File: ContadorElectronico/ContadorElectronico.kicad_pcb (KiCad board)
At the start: 2 copper layers, 60 x 90 mm, 24 parts, among them J1 INPUT, J2 POWER, SW1 MODE, SW2 INC, SW3 DEC, U1 LM358, U3 4N35, U4 4N35

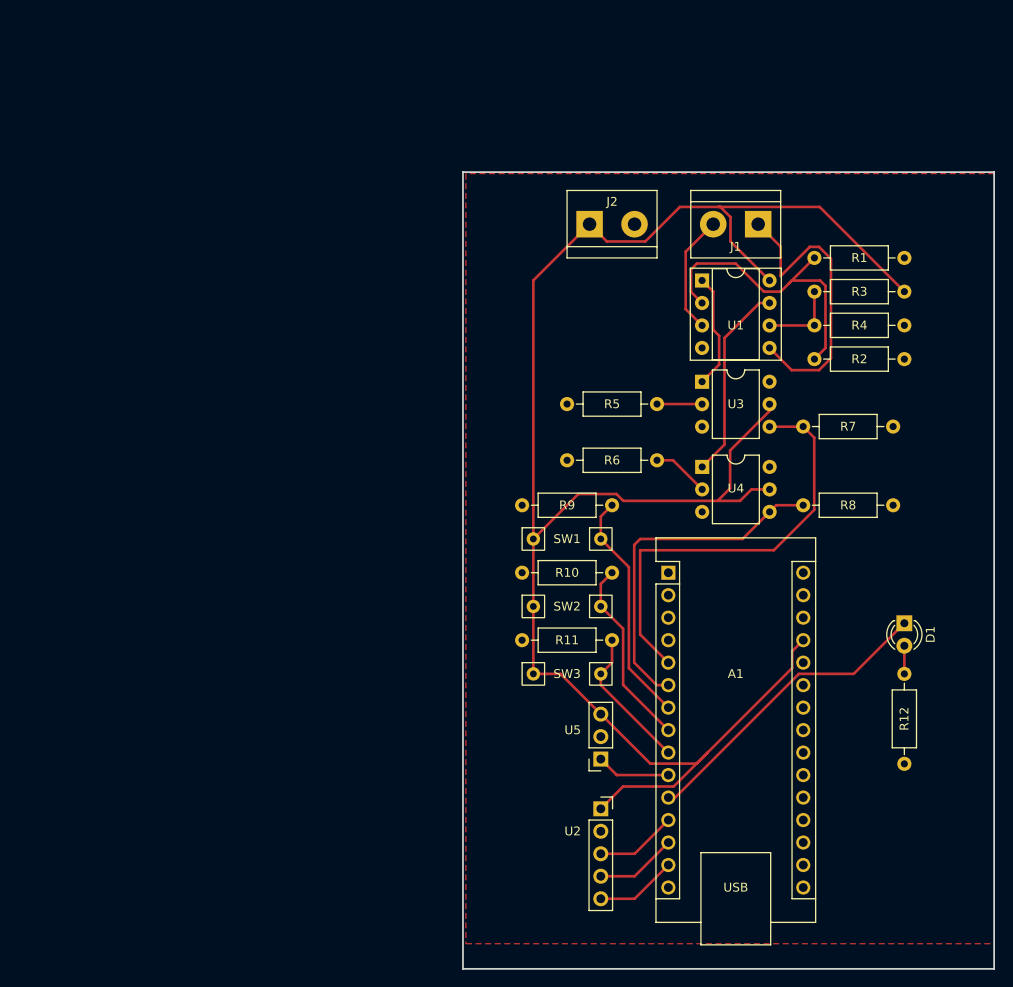
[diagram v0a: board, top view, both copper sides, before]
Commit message: PCB con tolerancias adecuadas
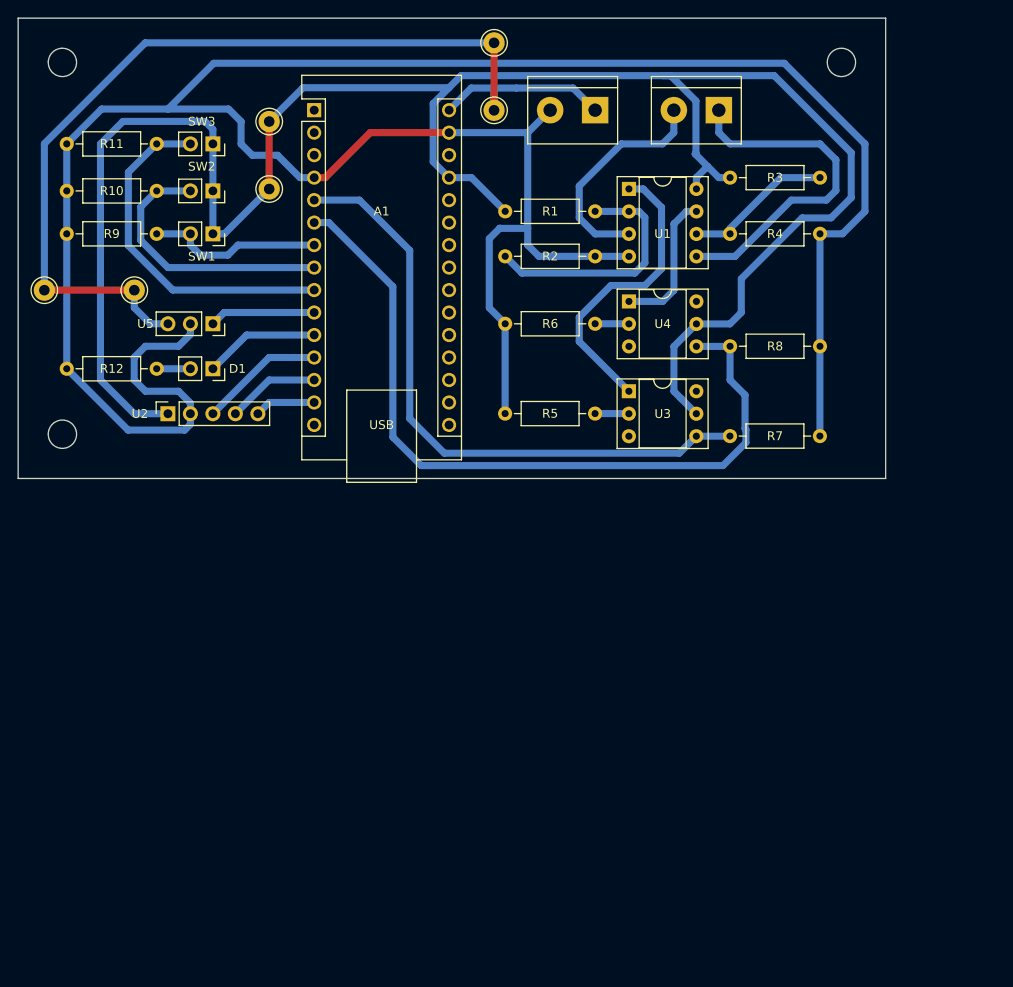
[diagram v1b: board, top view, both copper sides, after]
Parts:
- added J1: Conn_01x01_Pin, Connector_Pin:Pin_D1.0mm_L10.0mm_LooseFit, F.Cu at (52.7, 63.3)
- added J2: Conn_01x01_Pin, Connector_Pin:Pin_D1.0mm_L10.0mm_LooseFit, F.Cu at (62.9, 63.3)
- added J3: Conn_01x01_Pin, Connector_Pin:Pin_D1.0mm_L10.0mm_LooseFit, F.Cu at (103.5, 35.4)
- added J4: Conn_01x01_Pin, Connector_Pin:Pin_D1.0mm_L10.0mm_LooseFit, F.Cu at (103.5, 43.0)
- added J5: Conn_01x01_Pin, Connector_Pin:Pin_D1.0mm_L10.0mm_LooseFit, F.Cu at (78.1, 51.9)
- added J6: Conn_01x01_Pin, Connector_Pin:Pin_D1.0mm_L10.0mm_LooseFit, F.Cu at (78.1, 44.3)
- added REF**: MountingHole_3.2mm_M3, MountingHole:MountingHole_3.2mm_M3, F.Cu at (54.8, 37.6)
- added REF**: MountingHole_3.2mm_M3, MountingHole:MountingHole_3.2mm_M3, F.Cu at (142.8, 37.6)
- added REF**: MountingHole_3.2mm_M3, MountingHole:MountingHole_3.2mm_M3, F.Cu at (54.8, 79.6)
- D1: footprint LED_THT:LED_D3.0mm -> Connector_PinSocket_2.54mm:PinSocket_1x02_P2.54mm_Vertical
- SW1, SW2, SW3: footprint Custom:SW Header -> Connector_PinSocket_2.54mm:PinSocket_1x02_P2.54mm_Vertical
- U3, U4: footprint Package_DIP:DIP-6_W7.62mm -> Package_DIP:DIP-6_W7.62mm_Socket
- moved R12 91.2 mm to (65.4, 72.2), turned to 180 degrees
- moved D1 83.2 mm to (71.8, 72.2)
- moved R11 76.1 mm to (65.4, 46.8)
- moved SW3 72.0 mm to (71.8, 46.8), turned to -90 degrees
- moved R10 67.1 mm to (65.4, 52.1)
- moved U2 66.2 mm to (66.7, 77.3), turned to 90 degrees
- moved U5 65.9 mm to (71.8, 67.1), turned to -90 degrees
- moved A1 65.8 mm to (83.2, 43.0)
- moved SW2 61.7 mm to (71.8, 52.1), turned to -90 degrees
- moved R9 59.9 mm to (65.4, 57.0)
- moved SW1 52.8 mm to (71.8, 57.0), turned to -90 degrees
- moved R1 45.4 mm to (104.8, 54.4), turned to 0 degrees
- moved R2 36.8 mm to (104.8, 59.5)
- moved R3 23.5 mm to (130.2, 50.6), turned to 0 degrees
- moved U4 20.4 mm to (118.8, 64.6)
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- renumbered J1 to J7, J2 to J8
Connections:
- A1 pad 30: unconnected-(A1-VIN-Pad30) -> +9V
- J8 pad 1: +5V -> +9V
- U5 pad 3: +5V -> +9V
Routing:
- net GND: track 0.00 -> 298.9 mm
- net +9V: track 0.00 -> 117.5 mm
- net /RESET: track 39.1 -> 86.6 mm
- net +5V: track 205.4 -> 231.0 mm
- net /DEC: track 16.4 -> 39.7 mm
- net /MODE_LED: track 34.8 -> 13.0 mm
- net /COUNT: track 49.3 -> 70.7 mm
- net Net-(U1-Pad1): track 13.0 -> 33.7 mm
- net /COUNT_IN: track 13.5 -> 25.7 mm
- net /INC: track 21.5 -> 31.0 mm
- net Net-(U1B--): track 8.90 -> 17.0 mm
- net Net-(U1A--): track 34.7 -> 28.1 mm
- net /MODE: track 26.5 -> 20.0 mm
- net Net-(U1-Pad7): track 22.3 -> 16.2 mm
- net /RESET_IN: track 34.3 -> 39.4 mm
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- removed copper zone on F.Cu, net GND
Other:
- board size 60 x 90 mm -> 98 x 52 mm
